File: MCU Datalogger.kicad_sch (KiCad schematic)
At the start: 25 parts, among them U1 24LC1025, U2 24LC1025, U3 ATMEGA328P-AU, U4 DS1337S_, Y1 Crystal, Y2 Crystal

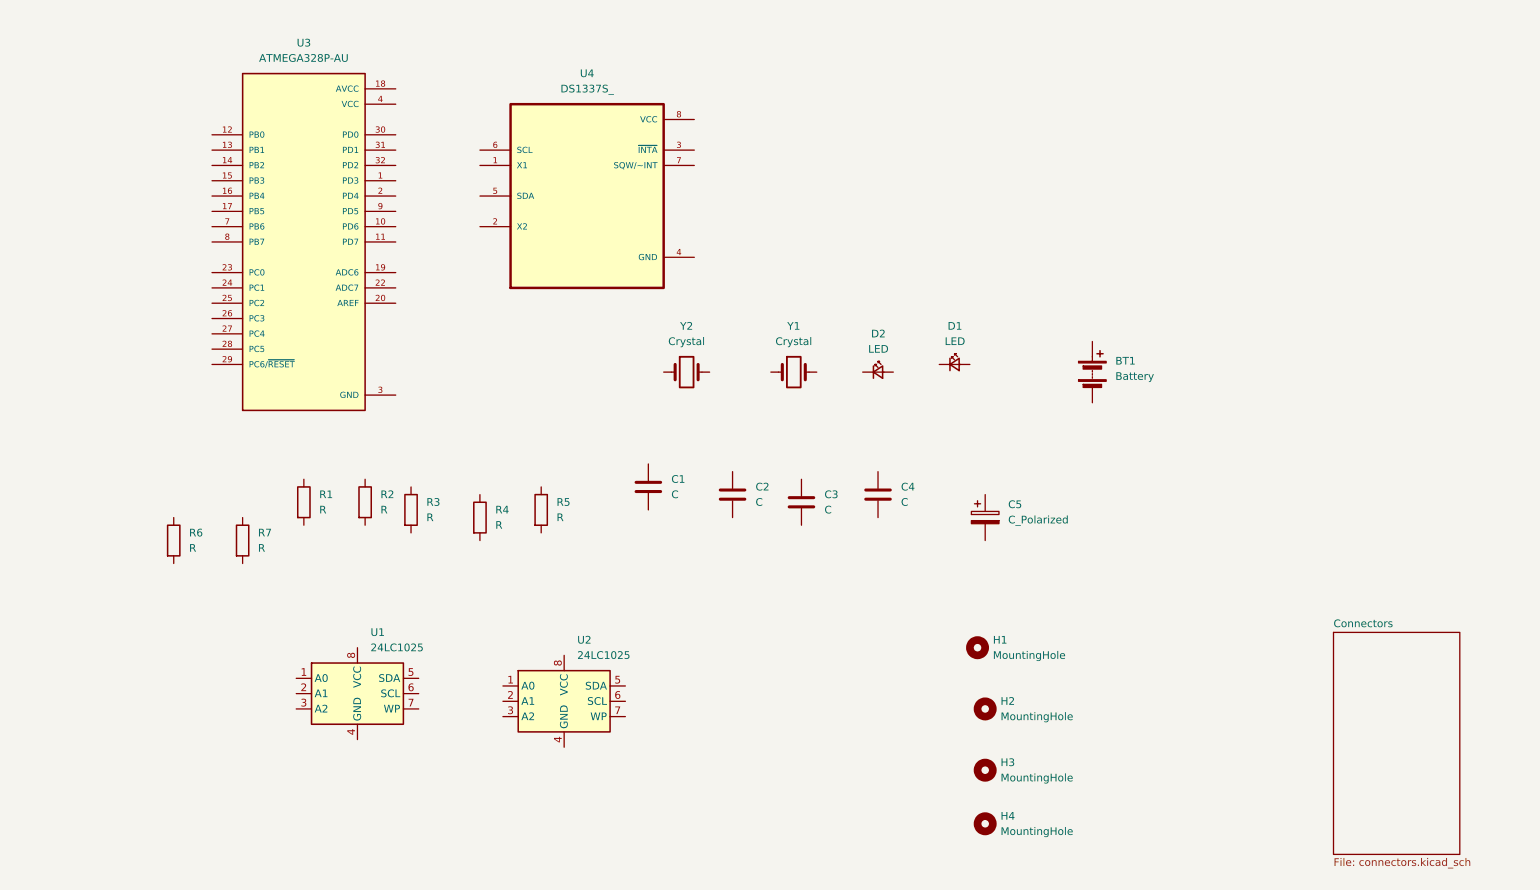
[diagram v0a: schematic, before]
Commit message: finish schema design
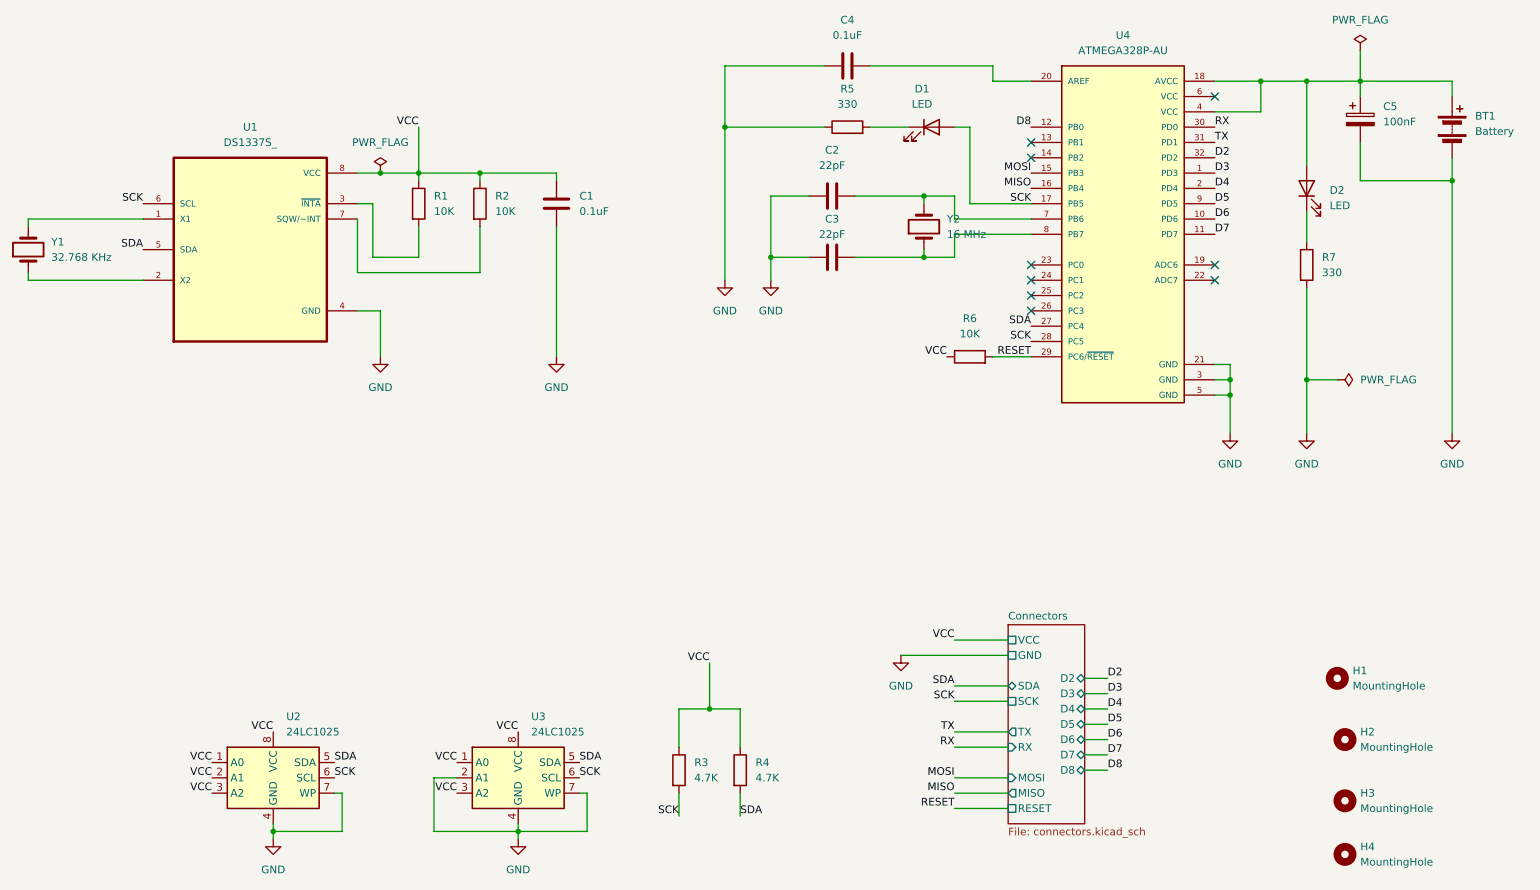
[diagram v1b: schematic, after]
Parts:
- BT1: footprint (none) -> Connector_PinHeader_2.54mm:PinHeader_2x01_P2.54mm_Vertical_SMD
- C1, C4: value C -> 0.1uF; footprint (none) -> Capacitor_SMD:C_0805_2012Metric
- C2: renamed from C3; value C -> 22pF; footprint (none) -> Capacitor_SMD:C_0805_2012Metric
- C3: renamed from C2; value C -> 22pF; footprint (none) -> Capacitor_SMD:C_0805_2012Metric
- C5: value C_Polarized -> 100nF; footprint (none) -> Capacitor_SMD:C_0805_2012Metric
- D1, D2: footprint SparkFun-LED:LED_0603_1608Metric -> LED_SMD:LED_0805_2012Metric; symbol SparkFun-LED:LED -> Device:LED
- H1, H2, H3, H4: footprint (none) -> MountingHole:MountingHole_2.1mm
- R1: renamed from R3; value R -> 10K; footprint (none) -> Resistor_SMD:R_0805_2012Metric
- R2: renamed from R4; value R -> 10K; footprint (none) -> Resistor_SMD:R_0805_2012Metric
- R3: renamed from R1; value R -> 4.7K; footprint (none) -> Resistor_SMD:R_0805_2012Metric
- R4: renamed from R2; value R -> 4.7K; footprint (none) -> Resistor_SMD:R_0805_2012Metric
- R5: renamed from R7; value R -> 330; footprint (none) -> Resistor_SMD:R_0805_2012Metric
- R6: value R -> 10K; footprint (none) -> Resistor_SMD:R_0805_2012Metric
- R7: renamed from R5; value R -> 330; footprint (none) -> Resistor_SMD:R_0805_2012Metric
- U2: renamed from U1; footprint (none) -> Package_SO:SOIC-8_5.3x5.3mm_P1.27mm
- U3: renamed from U2; footprint (none) -> Package_SO:SOIC-8_5.3x5.3mm_P1.27mm
- Y1: renamed from Y2; value Crystal -> 32.768 KHz; footprint (none) -> Crystal:Crystal_SMD_5032-2Pin_5.0x3.2mm_HandSoldering
- Y2: renamed from Y1; value Crystal -> 16 MHz; footprint (none) -> Crystal:Crystal_SMD_5032-2Pin_5.0x3.2mm_HandSoldering
- renumbered U4 to U1, U3 to U4
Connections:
- net GND: now also BT1.2 (-), C1.2, C2.1, C3.1, C4.1, C5.2, R5.1, R7.2, U1.4 (GND), U2.4 (GND), U2.7 (WP), U3.2 (A1), U3.4 (GND), U3.7 (WP)
- net VCC: now also C1.1, R1.1, R2.1, R3.1, R4.1, R6.1, U1.8 (VCC), U2.1 (A0), U2.2 (A1), U2.3 (A2), U2.8 (VCC), U3.1 (A0), U3.3 (A2), U3.8 (VCC); no longer U4.4 (VCC), U4.6 (VCC)
- net RESET: now reaches R6.2
- net RESET: now also U4.29 (PC6/~{RESET})
- net at C3.2: now also U4.8 (PB7), Y2.1
- net at D2.1 (K): now also R7.1
- net at D2.2 (A): now also BT1.1 (+), C5.1, U4.18 (AVCC), U4.4 (VCC)
- net at C2.2: now also U4.7 (PB6), Y2.2
- net SDA: now reaches U2.5 (SDA)
- net SDA: now also R4.2, U1.5 (SDA), U3.5 (SDA), U4.27 (PC4)
- net SCK: now reaches U2.6 (SCL)
- net SCK: now also D1.2 (A), R3.2, U1.6 (SCL), U3.6 (SCL), U4.17 (PB5), U4.28 (PC5)
- net at R1.2: now also U1.3 (~{INTA})
- net at Y1.1: now also U1.2 (X2)
- net at Y1.2: now also U1.1 (X1)
- net at R2.2: now also U1.7 (SQW/~INT)
- net at R5.2: now also D1.1 (K)
- net D3: now reaches U4.1 (PD3)
- net D6: now reaches U4.10 (PD6)
- net D7: now reaches U4.11 (PD7)
- net D8: now reaches U4.12 (PB0)
- net MOSI: now reaches U4.15 (PB3)
- net MISO: now reaches U4.16 (PB4)
- net D4: now reaches U4.2 (PD4)
- net at U4.20 (AREF): now also C4.2
- net RX: now reaches U4.30 (PD0)
- net TX: now reaches U4.31 (PD1)
- net D2: now reaches U4.32 (PD2)
- net D5: now reaches U4.9 (PD5)
- no-connect marks 0 -> 9
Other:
- sheet Connectors ports: added D2, D3, D4, D5, D6, D7, D8, GND, MISO, MOSI, RESET, RX, SCK, SDA, TX, VCC; removed none
- moved on the sheet: BT1, C1, C2, C3, C4, C5, D1, D2, H1, H2, H3, H4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
